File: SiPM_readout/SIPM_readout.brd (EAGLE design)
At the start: 160 x 100 mm, 27 parts

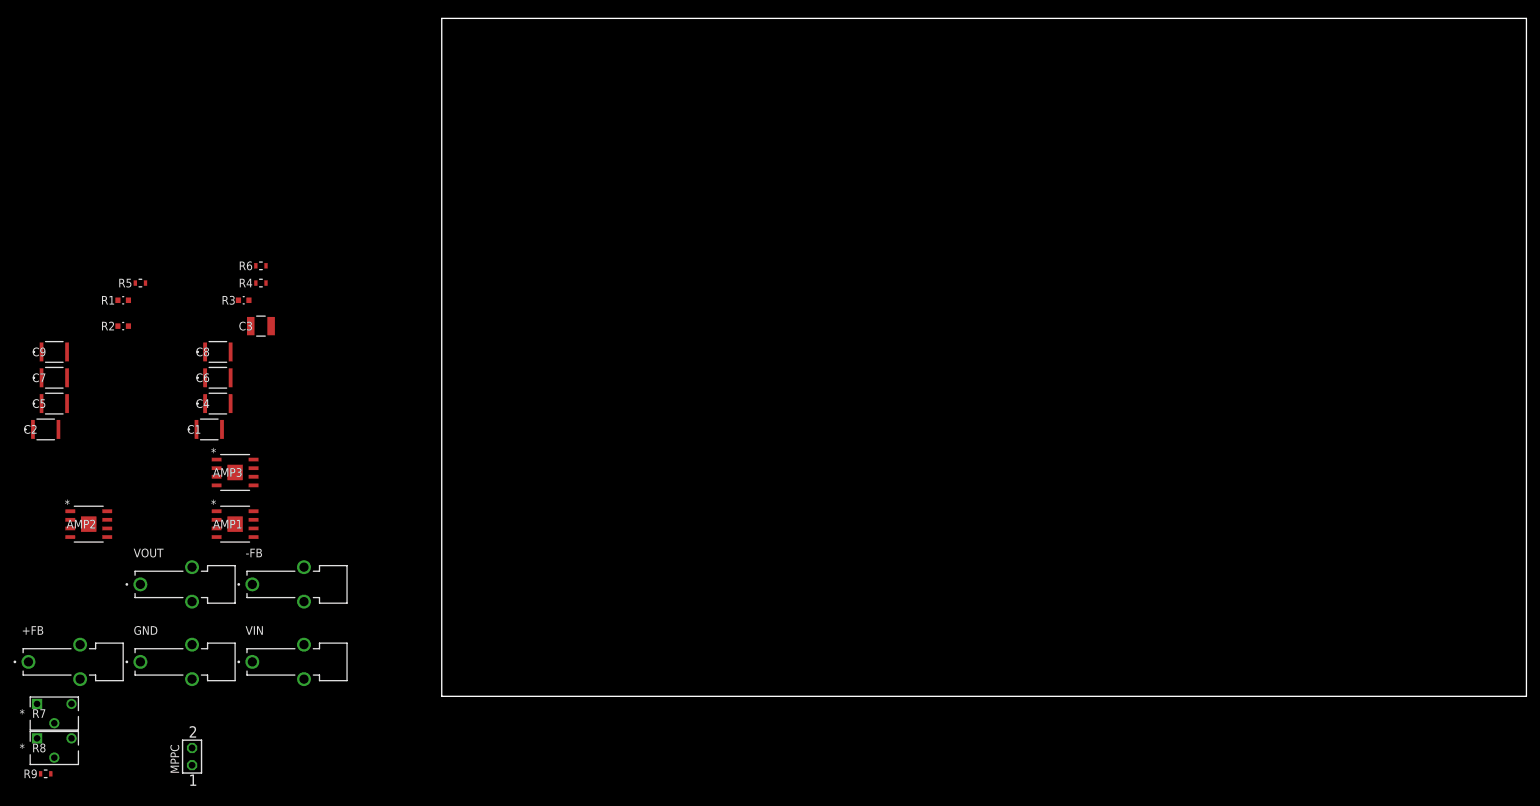
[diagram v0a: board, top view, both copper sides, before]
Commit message: mppc
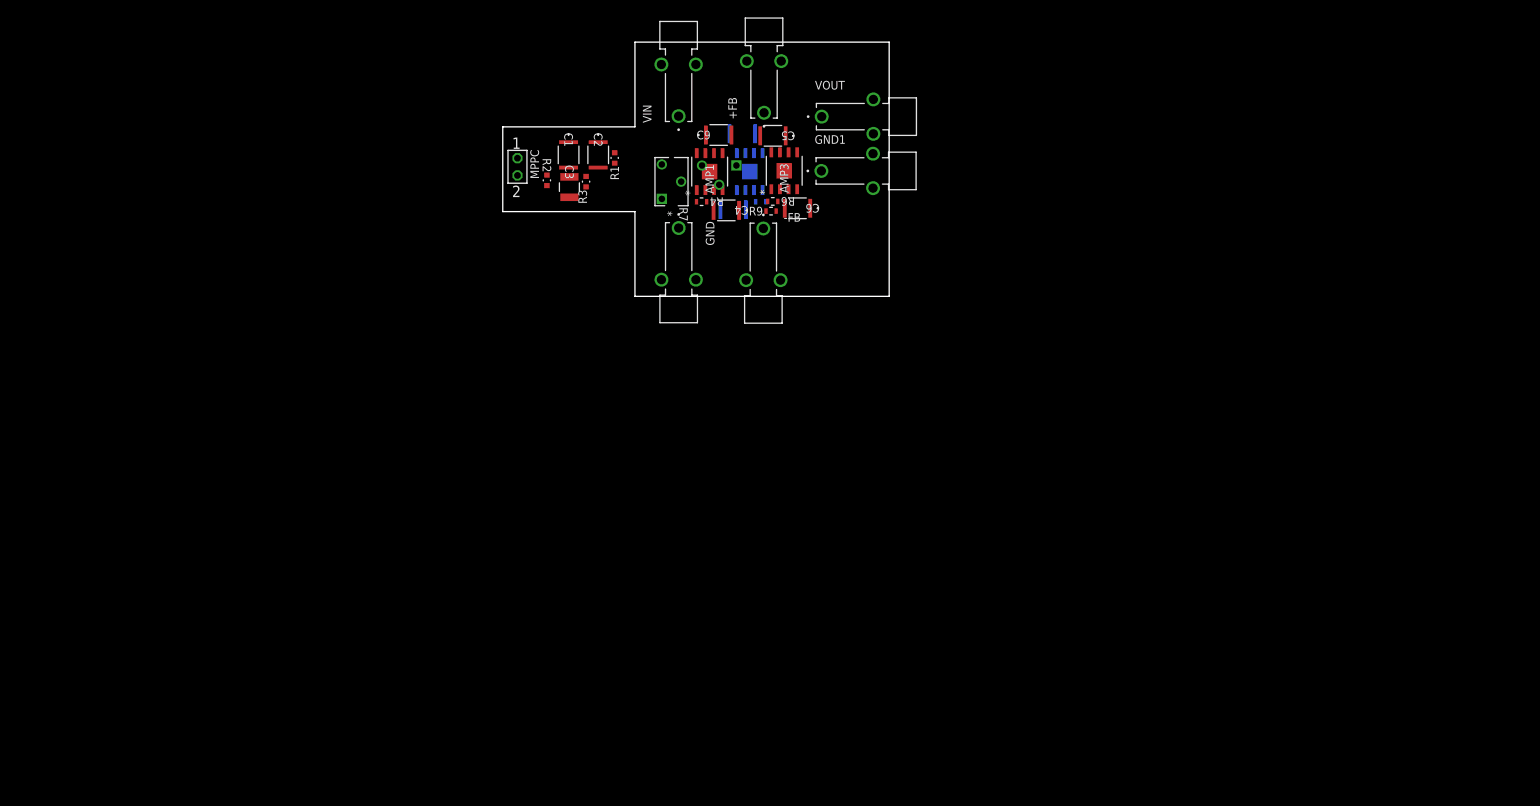
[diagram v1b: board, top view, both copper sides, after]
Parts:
- added GND1: 350180, SiPM_banana:TE_350180
- moved R9 135.4 mm to (48.6, 71.6)
- moved +FB 135.4 mm to (47.5, 86.1), turned to 90 degrees
- moved R8 125.7 mm to (38.4, 76.9), flipped to the bottom
- moved VOUT 121.9 mm to (56.0, 85.5)
- moved R7 120.0 mm to (33.9, 78.5), turned to 90 degrees
- moved C5 113.1 mm to (48.9, 82.7), turned to 180 degrees
- moved AMP2 110.5 mm to (45.4, 77.4), flipped to the bottom, turned to 90 degrees
- moved C7 107.7 mm to (44.4, 83.0), flipped to the bottom
- moved C9 103.1 mm to (40.9, 82.8)
- moved VIN 102.1 mm to (34.9, 85.6), turned to 90 degrees
- moved GND 102.0 mm to (35.0, 69.1), turned to 270 degrees
- moved MPPC 99.4 mm to (11.2, 78.1), turned to 180 degrees
- moved AMP3 92.4 mm to (50.5, 77.5), turned to 90 degrees
- moved R5 92.3 mm to (47.0, 73.0), flipped to the bottom, turned to 180 degrees
- moved -FB 91.9 mm to (47.4, 69.0), turned to 270 degrees
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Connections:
- removed net N$8: R8.2
- net GND: now also GND1.1
- net N$12: now also R8.2
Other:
- board size 160 x 100 mm -> 57 x 37.5 mm

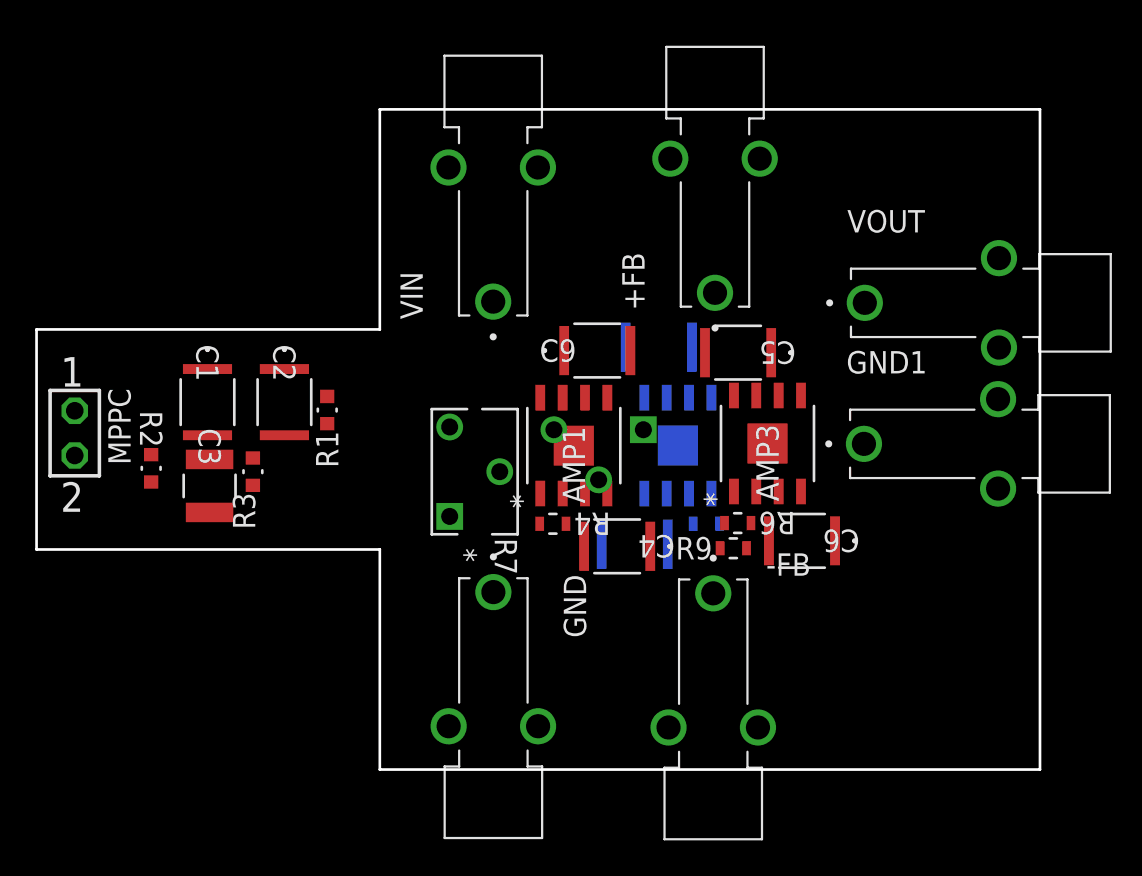
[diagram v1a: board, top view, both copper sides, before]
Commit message: mppc
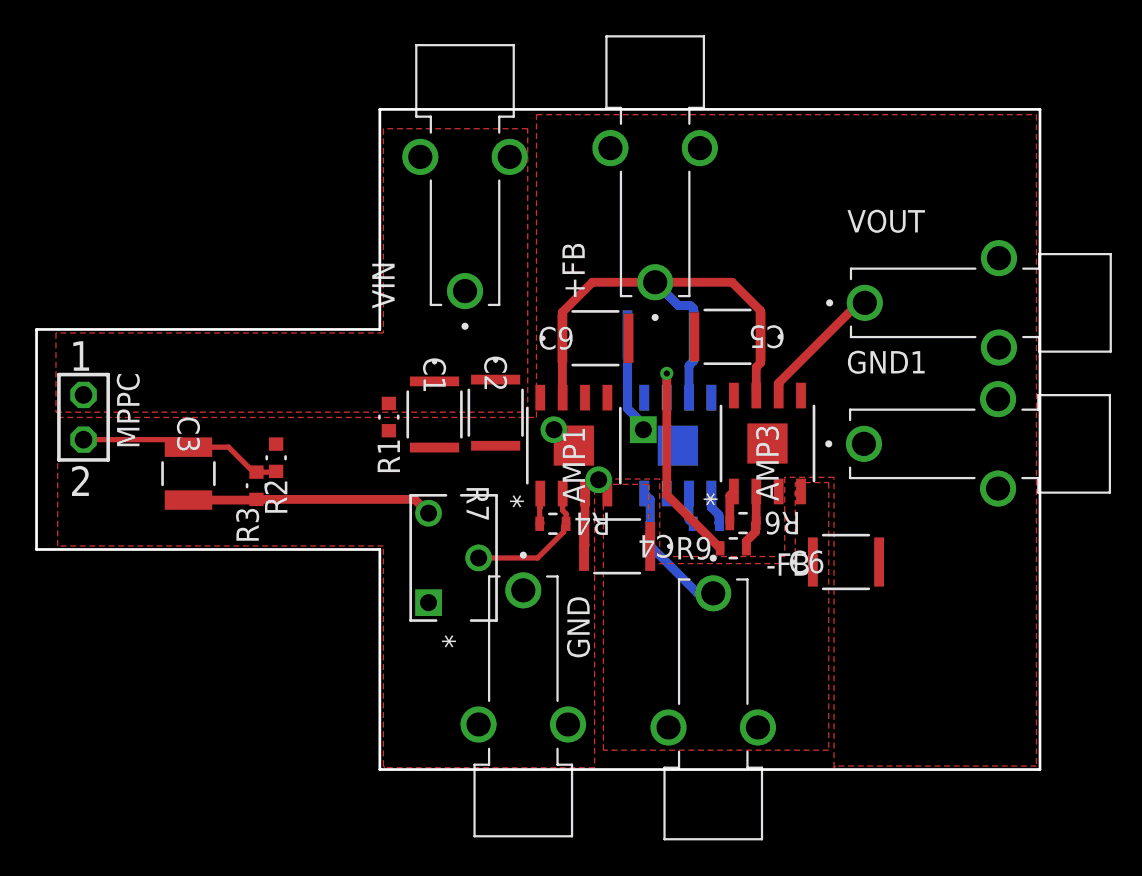
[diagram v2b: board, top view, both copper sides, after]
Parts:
- moved C1 12.9 mm to (31.6, 79.2)
- moved C2 12.0 mm to (35.1, 79.3)
- moved R2 7.13 mm to (22.6, 76.7), turned to 90 degrees
- moved R7 5.04 mm to (32.7, 73.6)
- moved R1 3.52 mm to (29.0, 79.0)
- moved +FB 3.45 mm to (44.1, 86.7)
- moved C6 2.77 mm to (55.0, 70.8), turned to 0 degrees
- moved VIN 1.71 mm to (33.3, 86.2)
- moved GND 1.70 mm to (36.6, 69.2)
- moved C3 1.39 mm to (17.6, 75.8)
- moved C5 1.08 mm to (48.2, 83.6)
- moved MPPC 1.03 mm to (11.7, 79.0)
- moved C8 1.00 mm to (42.0, 71.7), turned to 0 degrees
- moved R3 0.82 mm to (21.5, 75.1)
- moved C7 0.71 mm to (44.5, 83.7)
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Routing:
- net +FB: track 0.00 -> 30.7 mm
- net N$3: track 0.00 -> 14.0 mm
- net N$18: track 0.00 -> 12.6 mm, vias 0 -> 1
- net N$2: track 0.00 -> 11.8 mm
- net GND: track 0.00 -> 8.78 mm
- net -FB: track 0.00 -> 8.26 mm
- net N$4: track 0.00 -> 7.76 mm
- net VOUT: track 0.00 -> 7.49 mm
- net N$17: track 0.00 -> 3.46 mm
- net N$11: track 0.00 -> 1.91 mm
- net N$16: track 0.00 -> 1.89 mm
- net N$12: track 0.00 -> 1.81 mm
- net N$7: track 0.00 -> 1.78 mm
- added copper zone on layer 1, net -FB
- added copper zone on layer 1, net GND
- added copper zone on layer 1, net VIN
